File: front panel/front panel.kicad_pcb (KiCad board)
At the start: 2 copper layers, 30 x 39.6 mm, 0 parts

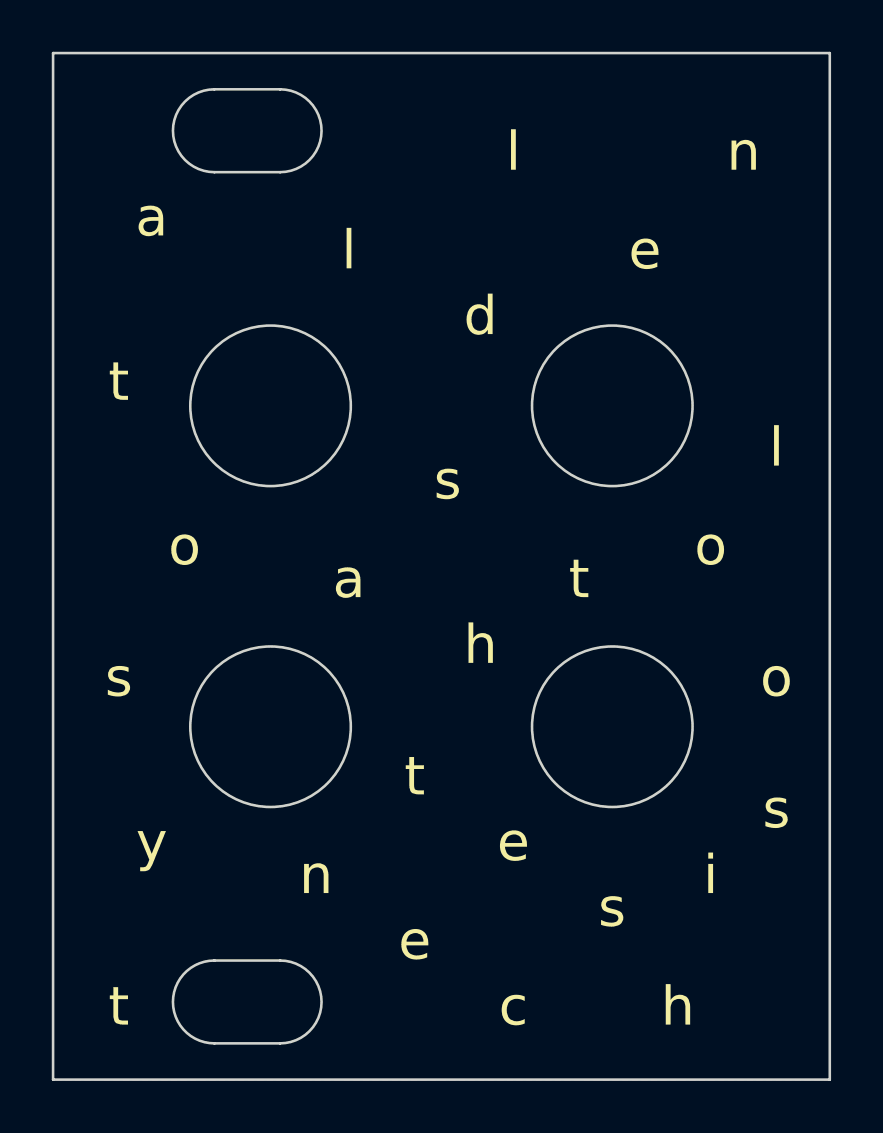
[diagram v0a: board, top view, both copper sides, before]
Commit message: kicad save, add panel, add passive protoboard, gerbers
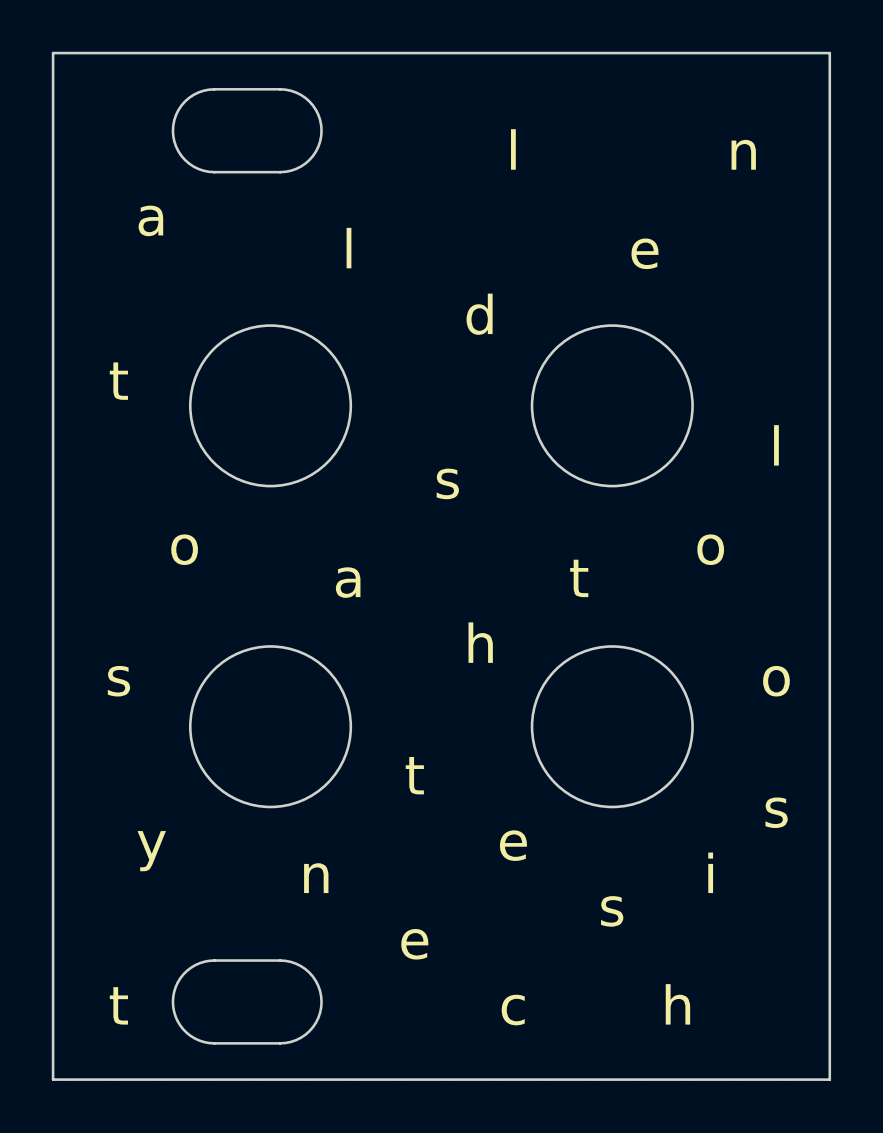
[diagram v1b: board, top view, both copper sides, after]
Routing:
- added copper zone on B.Cu, net (none)
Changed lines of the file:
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@@
       (outputformat 1)
       (mirror false)
-      (drillshape 1)
+      (drillshape 0)
       (scaleselection 1)
-      (outputdirectory "")
+      (outputdirectory "./")
     )
   )
@@
     (effects (font (size 1.5 1.5) (thickness 0.18)))
   )
-  (zone (net 0) (net_name "") (layer "F.Cu") (hatch edge 0.508)
+  (zone (net 0) (net_name "") (layers F&B.Cu) (hatch edge 0.508)
     (connect_pads (clearance 0.127))
     (min_thickness 0.254) (filled_areas_thickness no)
